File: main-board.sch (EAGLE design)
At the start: 1 part

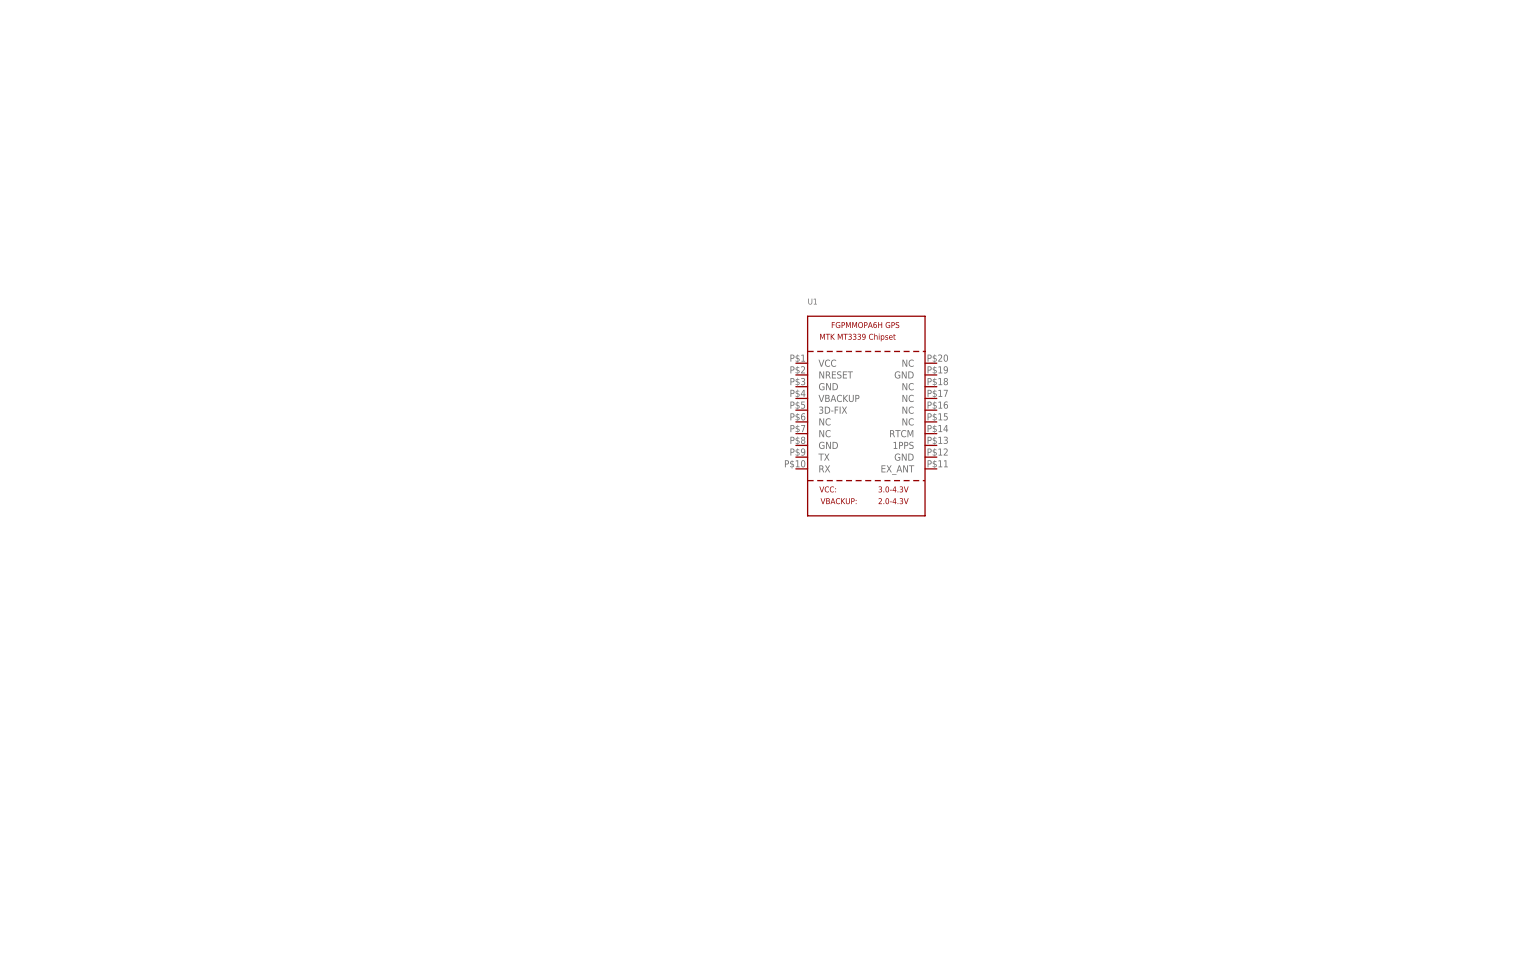
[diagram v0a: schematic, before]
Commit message: create power managment
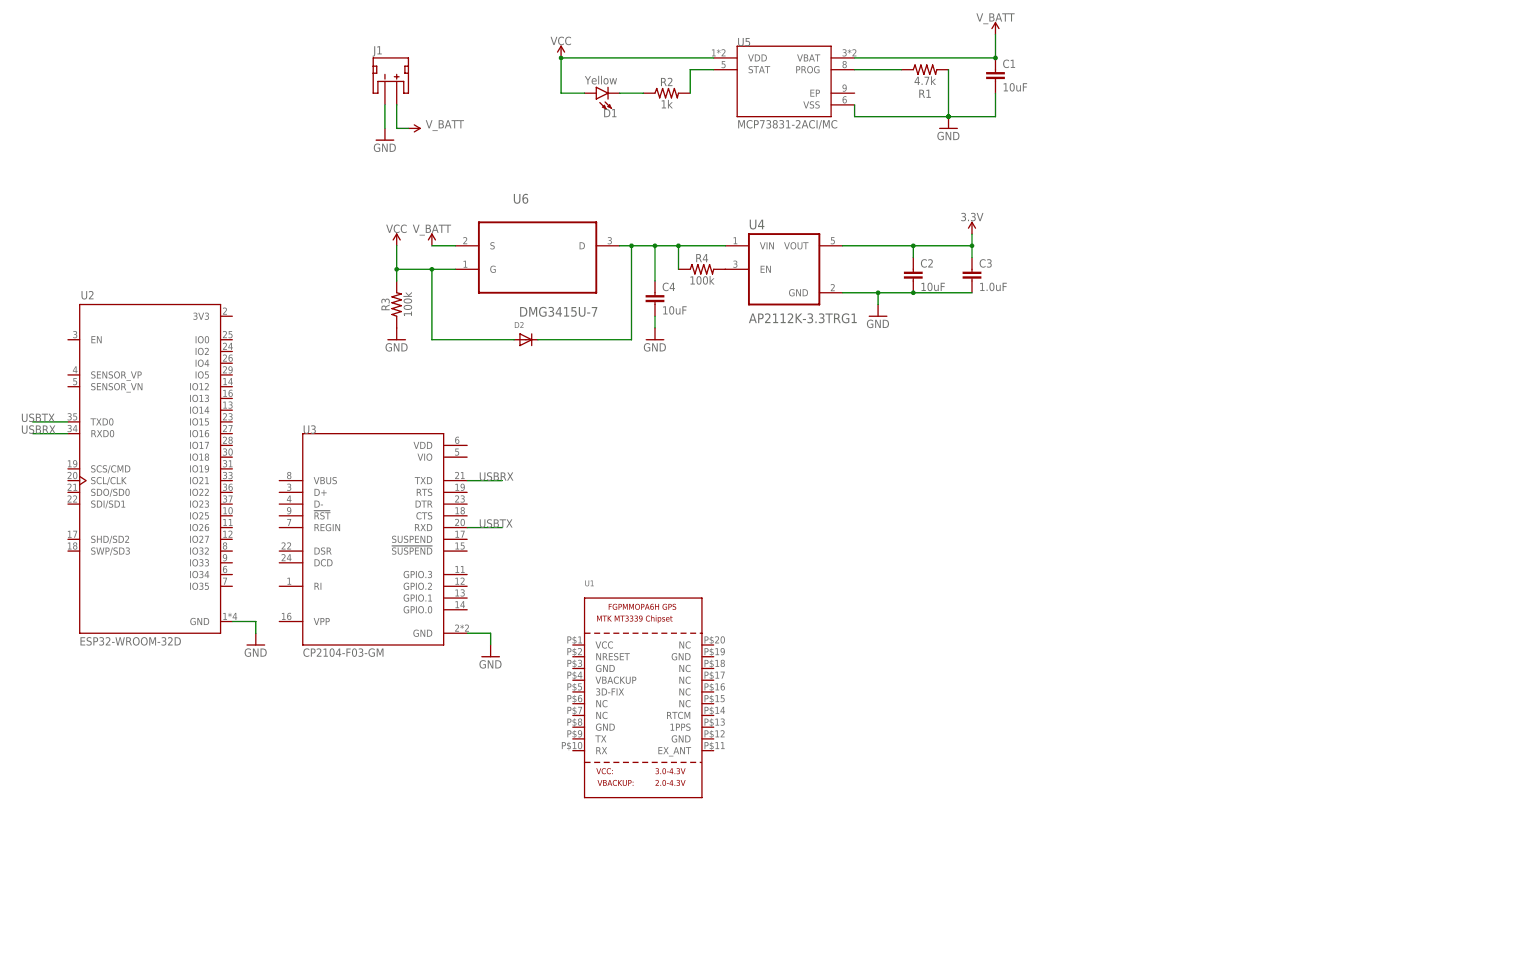
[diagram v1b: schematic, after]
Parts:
- added C1, C2, C4: 10uF, SparkFun-Capacitors:10UF-0805-10V-10%
- added C3: 1.0uF, SparkFun-Capacitors:1.0UF-0805-25V-(+80/-20%)
- added D1: Yellow, SparkFun-LED:LED-YELLOW0603
- added D2: (no value), adafruit:DIODESOD-123
- added J1: (no value), SparkFun-Connectors:JST_2MM_MALE
- added R1: 4.7k, SparkFun-Resistors:4.7KOHM-0603-1/10W-1%
- added R2: 1k, SparkFun-Resistors:1KOHM-0603-1/10W-1%
- added R3, R4: 100k, SparkFun-Resistors:100KOHM-0603-1/10W-1%
- added U2: ESP32-WROOM-32D, SnapEDA-Library:ESP32-WROOM-32D
- added U3: CP2104-F03-GM, SnapEDA-Library:CP2104-F03-GM
- added U4: AP2112K-3.3TRG1, SnapEDA-Library:AP2112K-3.3TRG1
- added U5: MCP73831-2ACI/MC, SnapEDA-Library:MCP73831-2ACI/MC
- added U6: DMG3415U-7, SnapEDA-Library:DMG3415U-7
- U1: OC_NEWARK (none) -> unknown
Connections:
- new net 3.3V: C2.1, C3.1, U4.VOUT
- new net GND: C1.2, C2.2, C3.2, C4.2, J1.-, R1.2, R3.1, U2.GND, U3.GND, U4.GND, U5.VSS
- new net N$1: R1.1, U5.PROG
- new net N$2: R2.2, U5.STAT
- new net N$3: D1.C, R2.1
- new net N$4: C4.1, D2.C, R4.1, U4.VIN, U6.D
- new net N$5: R4.2, U4.EN
- new net USBRX: U2.RXD0, U3.TXD
- new net USBTX: U2.TXD0, U3.RXD
- new net VCC: D1.A, D2.A, R3.2, U5.VDD, U6.G
- new net V_BATT: C1.1, J1.+, U5.VBAT, U6.S
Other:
- moved on the sheet: U1

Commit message: added board
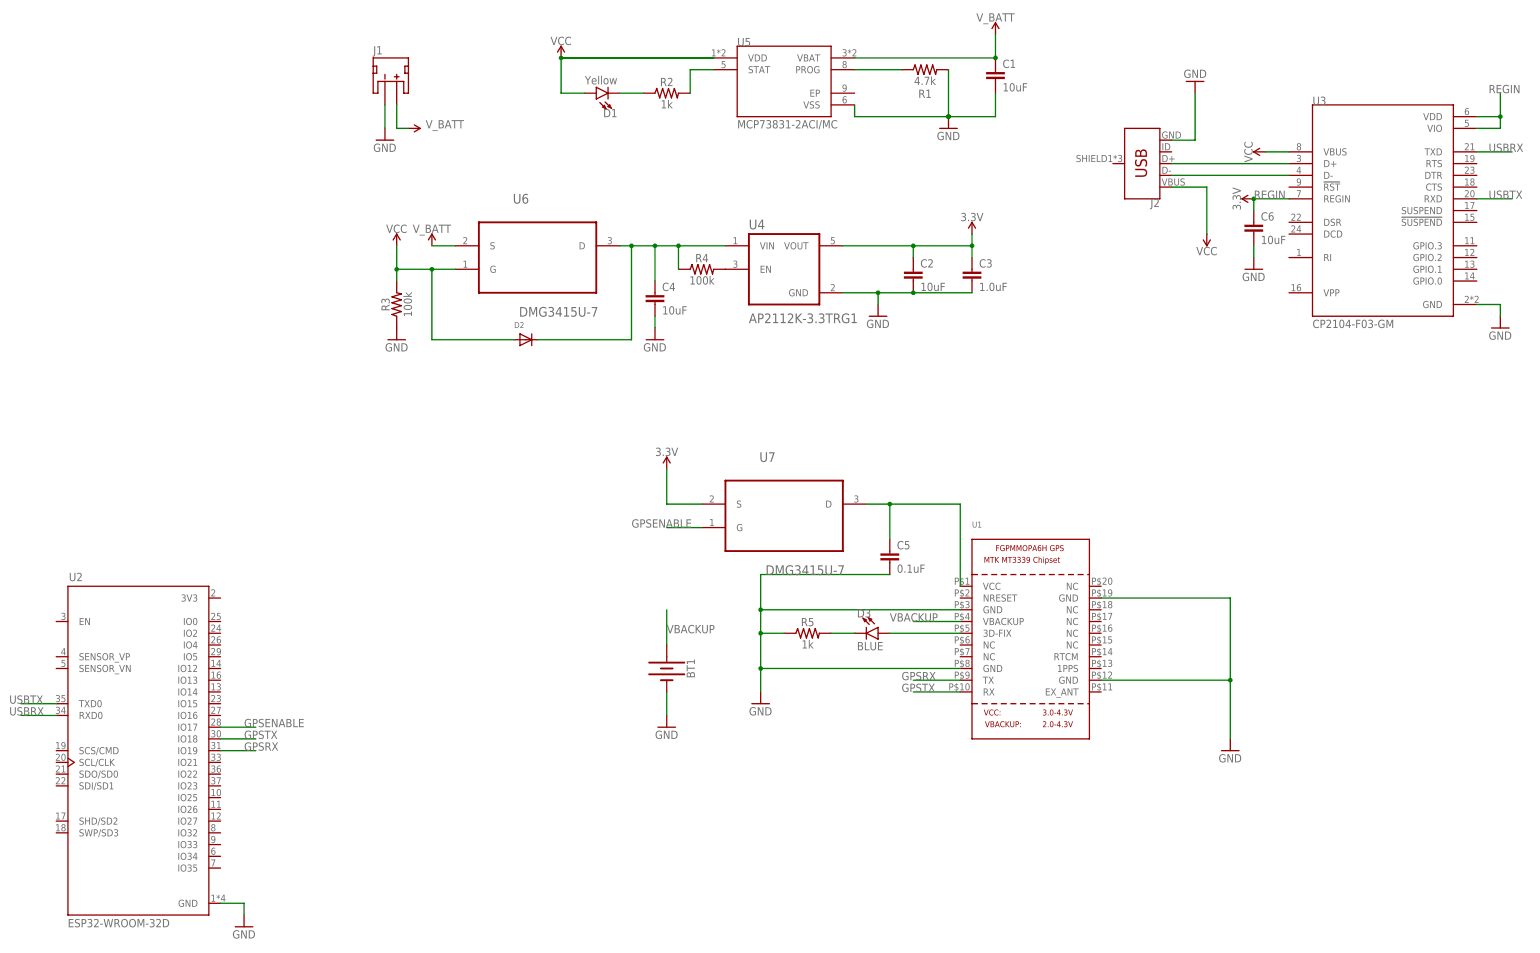
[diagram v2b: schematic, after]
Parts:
- added BT1: (no value), SparkFun-Batteries:BATTERY-20MM_PTH
- added C5: 0.1uF, SparkFun-Capacitors:0.1UF-0603-25V-(+80/-20%)
- added C6: 10uF, SparkFun-Capacitors:10UF-0805-10V-10%
- added D3: BLUE, SparkFun-LED:LED-BLUE0603
- added J2: (no value), SparkFun-Connectors:USB_MICRO-B_FEMALE-SMT
- added R5: 1k, SparkFun-Resistors:1KOHM-0603-1/10W-1%
- added U7: DMG3415U-7, SnapEDA-Library:DMG3415U-7
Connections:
- new net GPSENABLE: U2.IO17, U7.G
- new net GPSRX: U1.TX, U2.IO19
- new net GPSTX: U1.RX, U2.IO18
- new net N$10: J2.D-, U3.D-
- new net N$6: C5.1, U1.VCC, U7.D
- new net N$7: D3.A, U1.3D-FIX
- new net N$8: D3.C, R5.2
- new net N$9: J2.D+, U3.D+
- new net REGIN: C6.1, U3.REGIN, U3.VDD, U3.VIO
- new net VBACKUP: BT1.+, U1.VBACKUP
- net 3.3V: now also U7.S
- net GND: now also BT1.-, C5.2, C6.2, J2.GND, R5.1, U1.GND@1, U1.GND@2, U1.GND@3, U1.GND@4
- net VCC: now also J2.VBUS, U3.VBUS
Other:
- moved on the sheet: U1, U2, U3
